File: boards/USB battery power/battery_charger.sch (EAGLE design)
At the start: 2 parts, among them U1 MAX8934EETI+, U2 LTC3127EMSEPBF

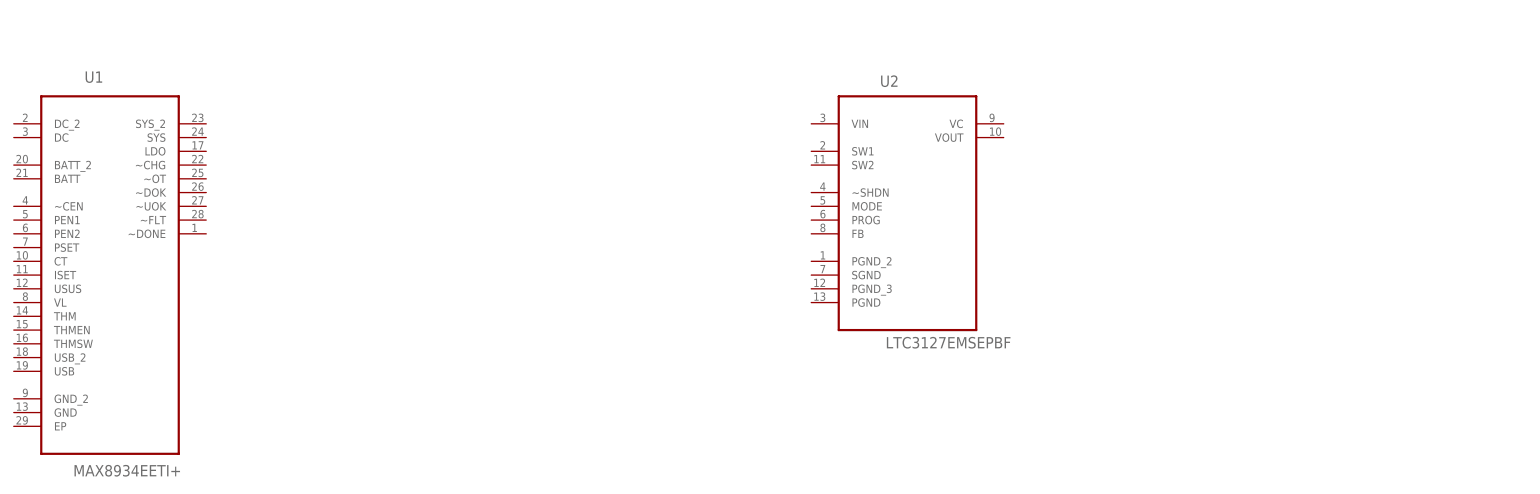
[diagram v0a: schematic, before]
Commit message: stuff
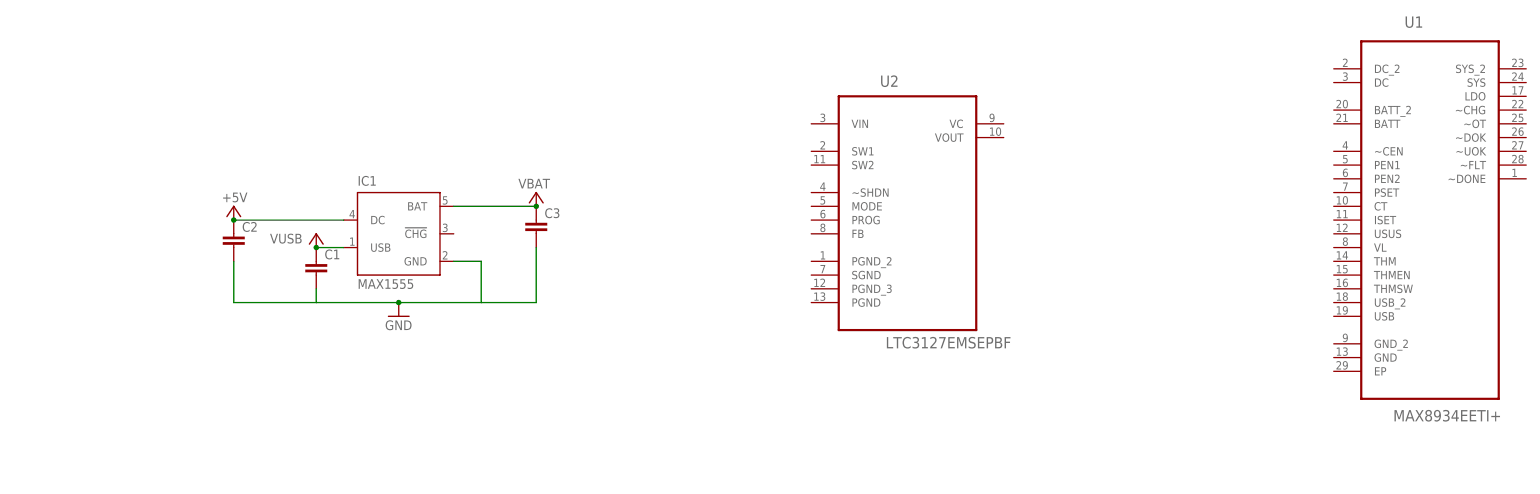
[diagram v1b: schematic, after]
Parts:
- added C1, C2, C3: (no value), rcl:C-EUC0603
- added IC1: MAX1555, Maxim:MAX1555
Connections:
- new net +5V: C2.1, IC1.DC
- new net +VBAT: C3.1, IC1.BAT
- new net +VUSB: C1.1, IC1.USB
- new net GND: C1.2, C2.2, C3.2, IC1.GND
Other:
- moved on the sheet: U1
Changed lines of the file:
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@@
 <layers>
 <layer number="1" name="Top" color="4" fill="1" visible="no" active="no"/>
+<layer number="2" name="Route2" color="1" fill="3" visible="no" active="no"/>
+<layer number="3" name="Route3" color="4" fill="3" visible="no" active="no"/>
+<layer number="4" name="Route4" color="1" fill="4" visible="no" active="no"/>
+<layer number="5" name="Route5" color="4" fill="4" visible="no" active="no"/>
+<layer number="6" name="Route6" color="1" fill="8" visible="no" active="no"/>
+<layer number="7" name="Route7" color="4" fill="8" visible="no" active="no"/>
+<layer number="8" name="Route8" color="1" fill="2" visible="no" active="no"/>
+<layer number="9" name="Route9" color="4" fill="2" visible="no" active="no"/>
+<layer number="10" name="Route10" color="1" fill="7" visible="no" active="no"/>
+<layer number="11" name="Route11" color="4" fill="7" visible="no" active="no"/>
+<layer number="12" name="Route12" color="1" fill="5" visible="no" active="no"/>
+<layer number="13" name="Route13" color="4" fill="5" visible="no" active="no"/>
+<layer number="14" name="Route14" color="1" fill="6" visible="no" active="no"/>
+<layer number="15" name="Route15" color="4" fill="6" visible="no" active="no"/>
 <layer number="16" name="Bottom" color="1" fill="1" visible="no" active="no"/>
 <layer number="17" name="Pads" color="2" fill="1" visible="no" active="no"/>
@@
 <part name="U1" library="Maxim" deviceset="MAX8934EETI+" device=""/>
 <part name="U2" library="LTC" deviceset="LTC3127EMSEPBF" device=""/>
+<part name="IC1" library="Maxim" deviceset="MAX1555" device=""/>
+<part name="C1" library="rcl" deviceset="C-EU" device="C0603"/>
+<part name="C2" library="rcl" deviceset="C-EU" device="C0603"/>
+<part name="C3" library="rcl" deviceset="C-EU" device="C0603"/>
+<part name="GND1" library="supply1" deviceset="GND" device=""/>
+<part name="U$1" library="Custom" deviceset="VBAT" device=""/>
+<part name="U$2" library="Custom" deviceset="VUSB" device=""/>
+<part name="P+1" library="supply1" deviceset="+5V" device=""/>
 </parts>
 <sheets>
@@
 </plain>
 <instances>
-<instance part="U1" gate="A" x="17.78" y="63.5"/>
+<instance part="U1" gate="A" x="261.62" y="73.66"/>
 <instance part="U2" gate="A" x="165.1" y="76.2"/>
+<instance part="IC1" gate="G$1" x="71.12" y="68.58"/>
+<instance part="C1" gate="G$1" x="55.88" y="63.5"/>
+<instance part="C2" gate="G$1" x="40.64" y="68.58"/>
+<instance part="C3" gate="G$1" x="96.52" y="71.12"/>
+<instance part="GND1" gate="1" x="71.12" y="53.34"/>
+<instance part="U$1" gate="G$1" x="96.52" y="73.66" smashed="yes">
+<attribute name="VALUE" x="99.06" y="78.74" size="1.778" layer="96" rot="R180"/>
+</instance>
+<instance part="U$2" gate="G$1" x="55.88" y="66.04" smashed="yes">
+<attribute name="VALUE" x="53.34" y="68.58" size="1.778" layer="96" rot="R180"/>
+</instance>
+<instance part="P+1" gate="1" x="40.64" y="73.66" smashed="yes">
+<attribute name="VALUE" x="43.18" y="76.2" size="1.778" layer="96" rot="R180"/>
+</instance>
 </instances>
 <busses>
 </busses>
 <nets>
+<net name="GND" class="0">
+<segment>
+<pinref part="IC1" gate="G$1" pin="GND"/>
+<wire x1="81.28" y1="63.5" x2="86.36" y2="63.5" width="0.1524" layer="91"/>
+<wire x1="86.36" y1="63.5" x2="86.36" y2="55.88" width="0.1524" layer="91"/>
+<pinref part="C1" gate="G$1" pin="2"/>
+<wire x1="86.36" y1="55.88" x2="71.12" y2="55.88" width="0.1524" layer="91"/>
+<wire x1="71.12" y1="55.88" x2="55.88" y2="55.88" width="0.1524" layer="91"/>
+<wire x1="55.88" y1="55.88" x2="55.88" y2="58.42" width="0.1524" layer="91"/>
+<pinref part="C2" gate="G$1" pin="2"/>
+<wire x1="55.88" y1="55.88" x2="40.64" y2="55.88" width="0.1524" layer="91"/>
+<wire x1="40.64" y1="55.88" x2="40.64" y2="63.5" width="0.1524" layer="91"/>
+<pinref part="C3" gate="G$1" pin="2"/>
+<wire x1="96.52" y1="66.04" x2="96.52" y2="55.88" width="0.1524" layer="91"/>
+<wire x1="96.52" y1="55.88" x2="86.36" y2="55.88" width="0.1524" layer="91"/>
+<pinref part="GND1" gate="1" pin="GND"/>
+<junction x="71.12" y="55.88"/>
+</segment>
+</net>
+<net name="+VBAT" class="0">
+<segment>
+<pinref part="IC1" gate="G$1" pin="BAT"/>
+<pinref part="C3" gate="G$1" pin="1"/>
+<wire x1="81.28" y1="73.66" x2="96.52" y2="73.66" width="0.1524" layer="91"/>
+<pinref part="U$1" gate="G$1" pin="+VBAT"/>
+<junction x="96.52" y="73.66"/>
+</segment>
+</net>
+<net name="+VUSB" class="0">
+<segment>
+<pinref part="C1" gate="G$1" pin="1"/>
+<pinref part="IC1" gate="G$1" pin="USB"/>
+<wire x1="55.88" y1="66.04" x2="60.96" y2="66.04" width="0.1524" layer="91"/>
+<pinref part="U$2" gate="G$1" pin="+VUSB"/>
+<junction x="55.88" y="66.04"/>
+</segment>
+</net>
+<net name="+5V" class="0">
+<segment>
+<pinref part="C2" gate="G$1" pin="1"/>
+<pinref part="IC1" gate="G$1" pin="DC"/>
+<wire x1="40.64" y1="71.12" x2="60.96" y2="71.12" width="0.1524" layer="91"/>
+<pinref part="P+1" gate="1" pin="+5V"/>
+<junction x="40.64" y="71.12"/>
+</segment>
+</net>
 </nets>
 </sheet>
